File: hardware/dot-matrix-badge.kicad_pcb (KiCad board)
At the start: 2 copper layers, 55 x 20 mm, 11 parts, among them J1 AVR-UPDI-6, SW1 SW_SPST, SW2 SW_Push, SW3 SW_Push, U1 ATtiny1604-SS

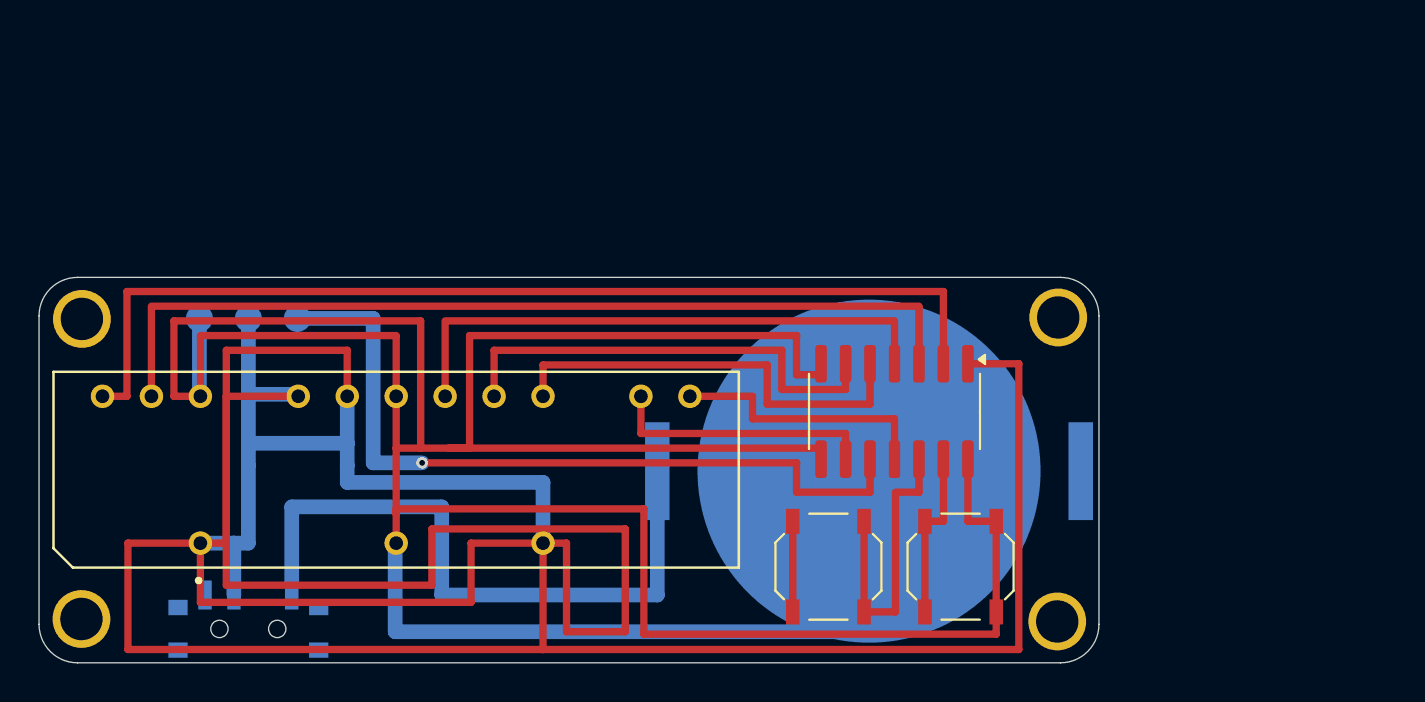
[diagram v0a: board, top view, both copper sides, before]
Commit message: pcb payout almost complete
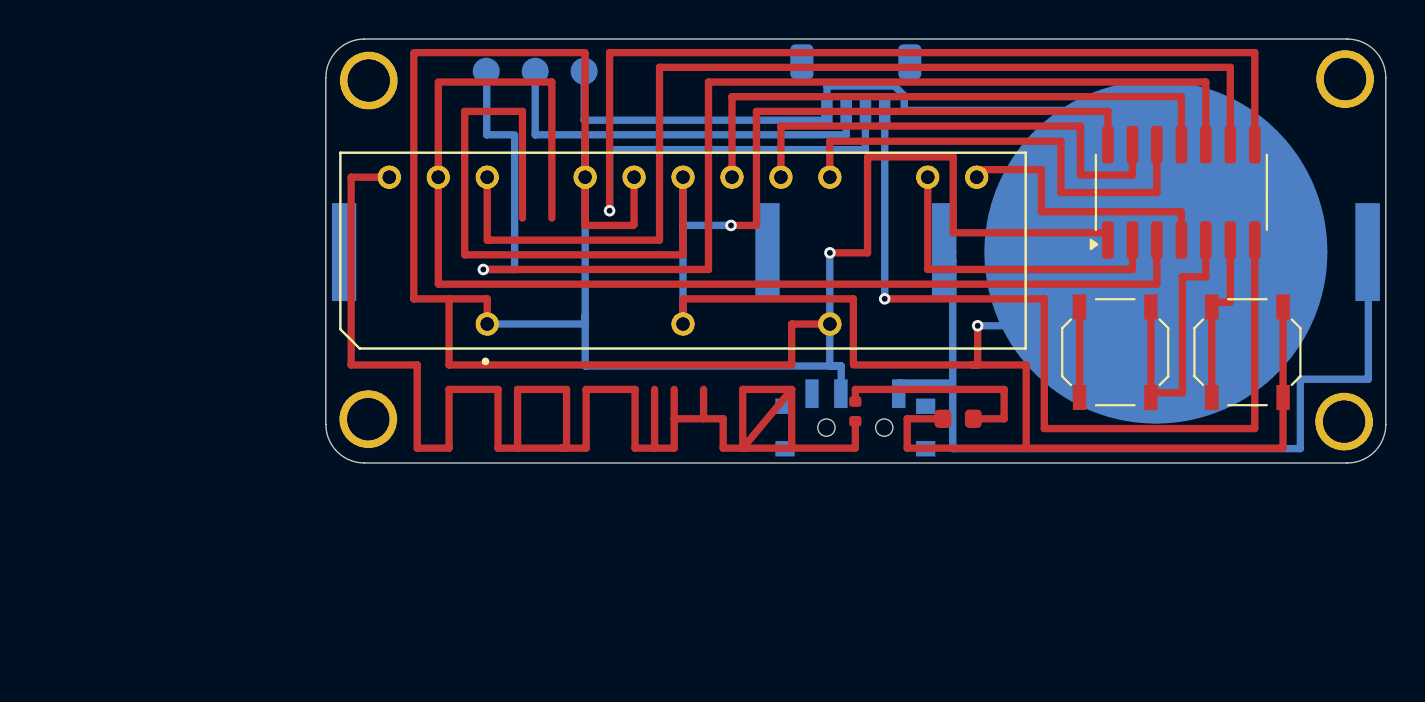
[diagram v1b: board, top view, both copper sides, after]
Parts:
- added BT2: Battery_Cell, DotMatrixBadge:SpareBatteryHolder_Keystone_3034_1x20mm, B.Cu at (54.8, 28.7)
- added D2: LED, LED_SMD:LED_0603_1608Metric, F.Cu at (75.7, 37.3)
- added J2: JST_04, Connector_JST:JST_SH_BM04B-SRSS-TB_1x04-1MP_P1.00mm_Vertical, B.Cu at (70.4, 20.0)
- added R1: 1k, Resistor_SMD:R_0402_1005Metric, F.Cu at (70.4, 37.0)
- moved SW1 33.2 mm to (70.4, 37.5)
- moved H1 19.4 mm to (45.1, 19.8)
- moved H3 19.4 mm to (95.8, 19.7)
- moved BT1 18.7 mm to (86.0, 28.7)
- moved D1 18.7 mm to (61.4, 28.6)
- moved U1 18.7 mm to (87.3, 25.6), turned to 90 degrees
- moved SW2 18.6 mm to (83.8, 33.9)
- moved SW3 18.6 mm to (90.7, 33.9)
- moved H4 18.1 mm to (95.7, 37.5)
- moved H2 18.1 mm to (45.1, 37.4)
- moved J1 16.1 mm to (51.2, 19.3), turned to 0 degrees
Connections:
- D1 pad 24: GND -> RESET
- U1 pad 11: DIN -> BL
- U1 pad 12: BTN1 -> CLK
- U1 pad 13: BTN2 -> CE
- U1 pad 2: DOUT -> RS
- U1 pad 4: BL -> DIN
- U1 pad 5: CLK -> BTN1
- U1 pad 6: CE -> BTN2
- U1 pad 7: GND -> SCL
- U1 pad 8: GND -> SDA
- U1 pad 9: RS -> RESET
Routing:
- net VCC: track 216.3 -> 149.6 mm, vias 0 -> 1
- net SDA: track 0.00 -> 64.9 mm, vias 0 -> 1
- net RESET: track 0.00 -> 54.9 mm
- net SCL: track 0.00 -> 45.5 mm, vias 0 -> 1
- net DOUT: track 52.8 -> 86.7 mm
- net UPDI: track 40.5 -> 63.9 mm
- net OSC: track 47.4 -> 62.9 mm
- net Net-(BT1-+): track 34.1 -> 45.8 mm
- net Net-(D2-A): track 0.00 -> 11.5 mm
- net GND: track 193.7 -> 198.0 mm, vias 0 -> 2
- net RS: track 13.9 -> 16.9 mm
- net CLK: track 22.7 -> 24.0 mm
- net DIN: track 13.8 -> 14.9 mm
- net CE: track 24.0 -> 25.0 mm
- net BL: track 29.2 -> 30.0 mm
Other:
- board size 55 x 20 mm -> 55 x 22 mm
